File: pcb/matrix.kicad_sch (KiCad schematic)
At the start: 140 parts, among them SW1 ESC, SW10 9, SW11 0, SW12 -, SW13 =, SW14 BACK, SW15 ROTARY, SW16 TAB, SW17 Q, SW18 W, SW19 E, SW2 1, SW20 R, SW21 T, SW22 Y, SW23 U, SW24 I, SW25 O, SW26 P, SW27 [, SW28 ], SW29 \, SW3 2, SW30 PgUp, SW31 CAPS, SW32 A, SW33 S, SW34 D, SW35 F, SW36 G, SW37 H, SW38 J, SW39 K, SW4 3, SW40 L, SW41 ;, SW42 ', SW43 ENTER, SW44 PgDn, SW45 LSHIFT, SW46 Z, SW47 X, SW48 C, SW49 V, SW5 4, SW50 B, SW51 N, SW52 M, SW53 ,, SW54 ., SW55 /, SW56 RSHIFT, SW57 UP, SW58 HOME, SW59 CTRL, SW6 5, SW60 SUPER, SW61 ALT, SW62 SPACE, SW63 FN2, SW64 FN1, SW65 LEFT, SW66 DOWN, SW67 RIGHT, SW68 RALT, SW7 6, SW8 7, SW9 8

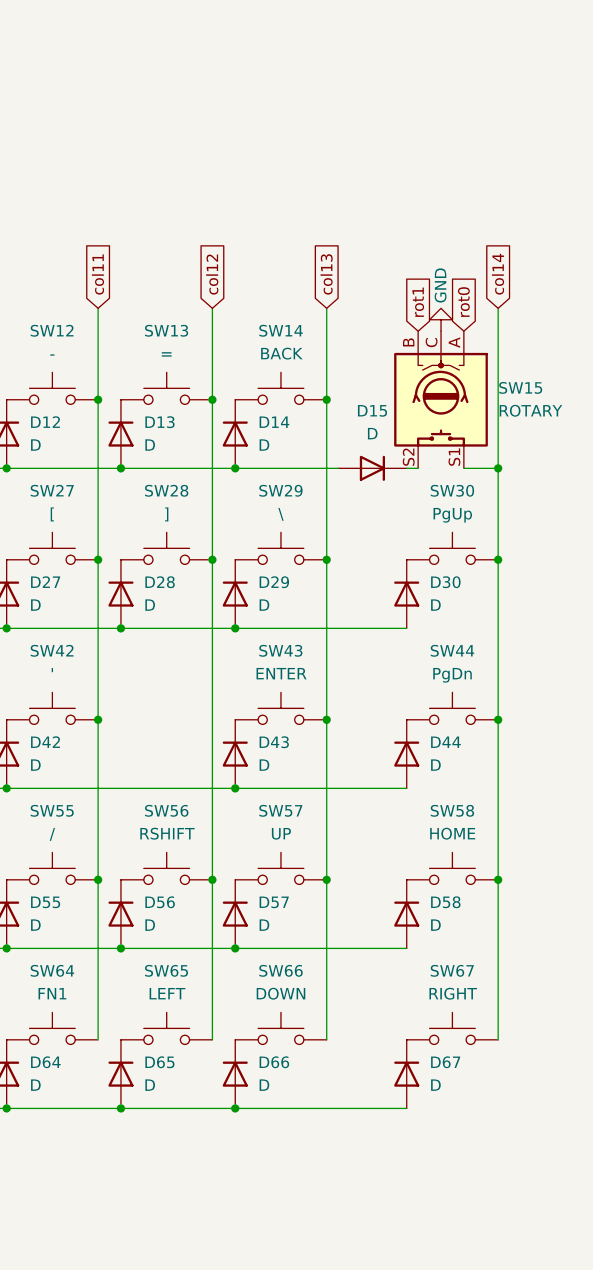
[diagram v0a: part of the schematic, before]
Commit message: JLCPCB 1
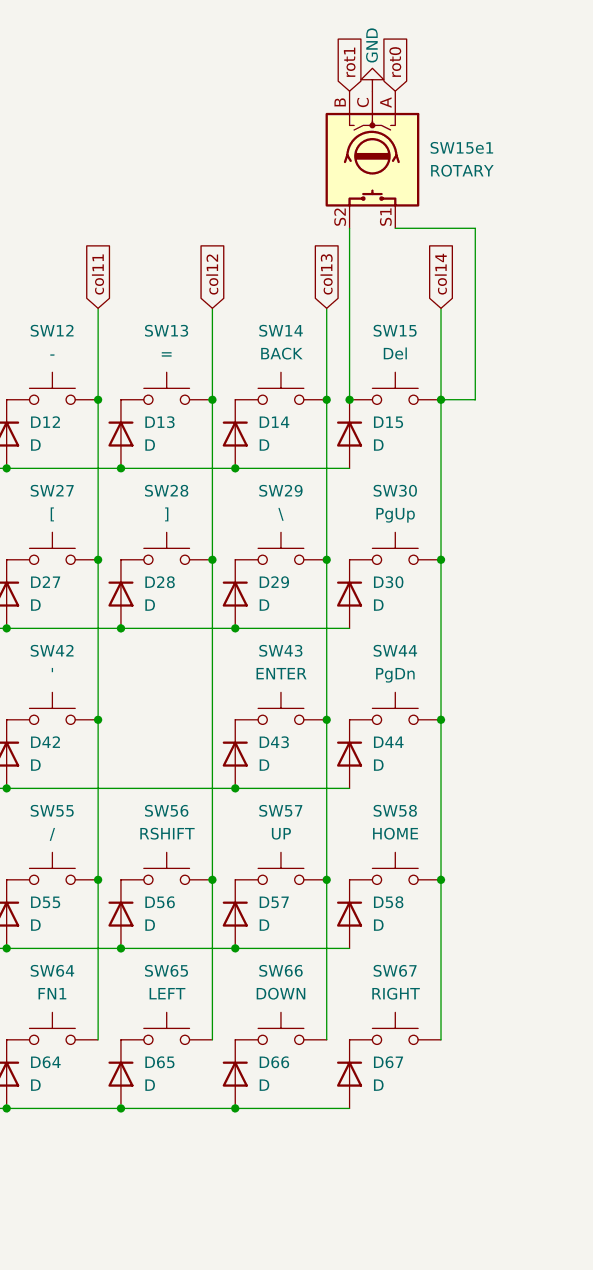
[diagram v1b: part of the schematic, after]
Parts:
- added SW15: Del, PCM_marbastlib-mx:SW_MX_HS_CPG151101S11_1u, symbol Switch:SW_Push
- renumbered SW15 to SW15e1
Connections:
- net col14: now also SW15.2
- net at D15.1 (K), SW15e1.S2: now also SW15.1
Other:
- moved on the sheet: D15, D30, D44, D58, D67, SW15e1, SW30, SW44, SW58, SW67
